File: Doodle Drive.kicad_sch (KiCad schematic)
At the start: 38 parts, among them J1 USB_B, J2 PINHD_1x4_Male, J3 Screw_Terminal_01x02, J6 PINHD_1x2_Male, J9 PINHD_1x3_Male, U1 STM32F411RETx, U6 AP7343-33W5-7, U7 CP2102-GMR, Y1 32.768KHz ±20ppm 12.5pF, Y2 25MHZ 12PF

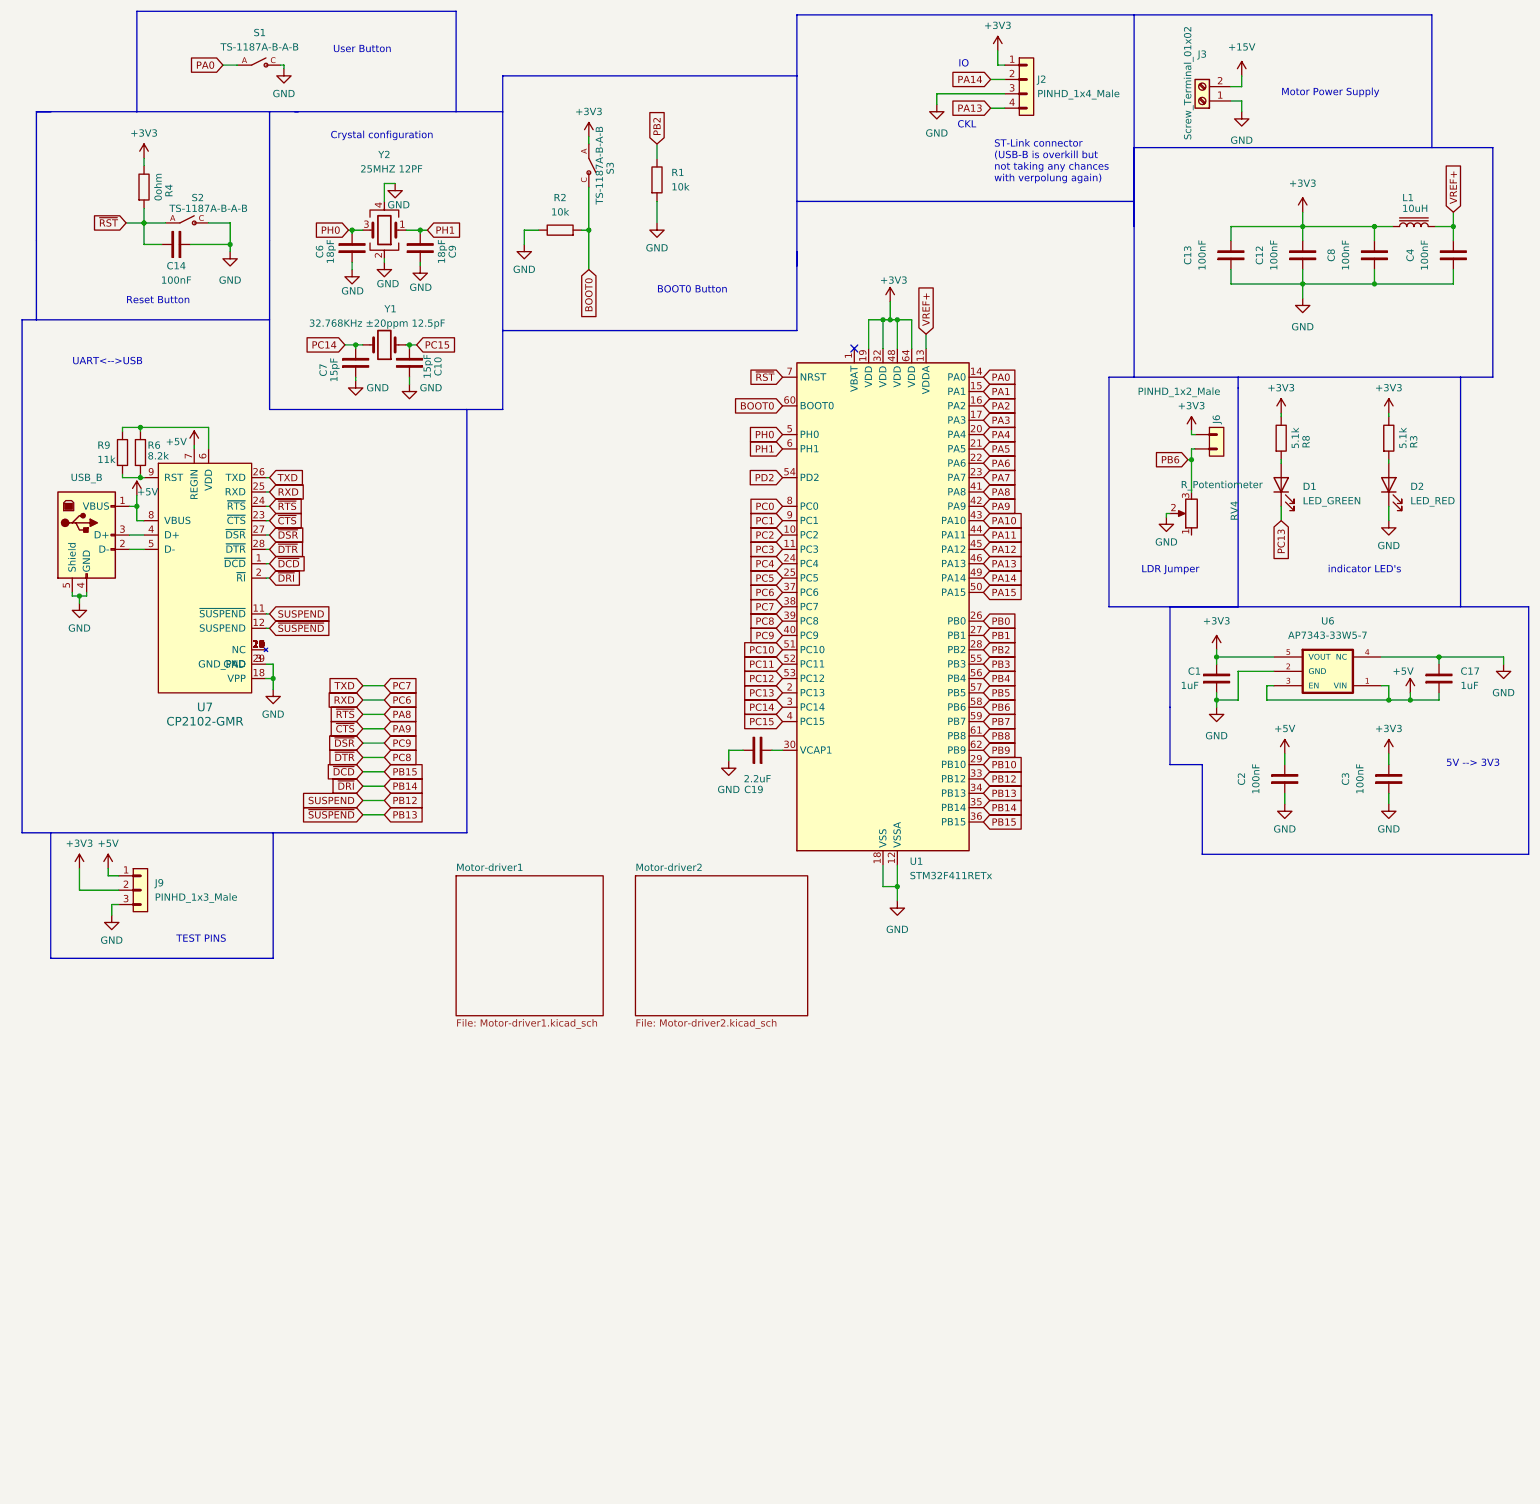
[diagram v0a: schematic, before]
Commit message: letzter code
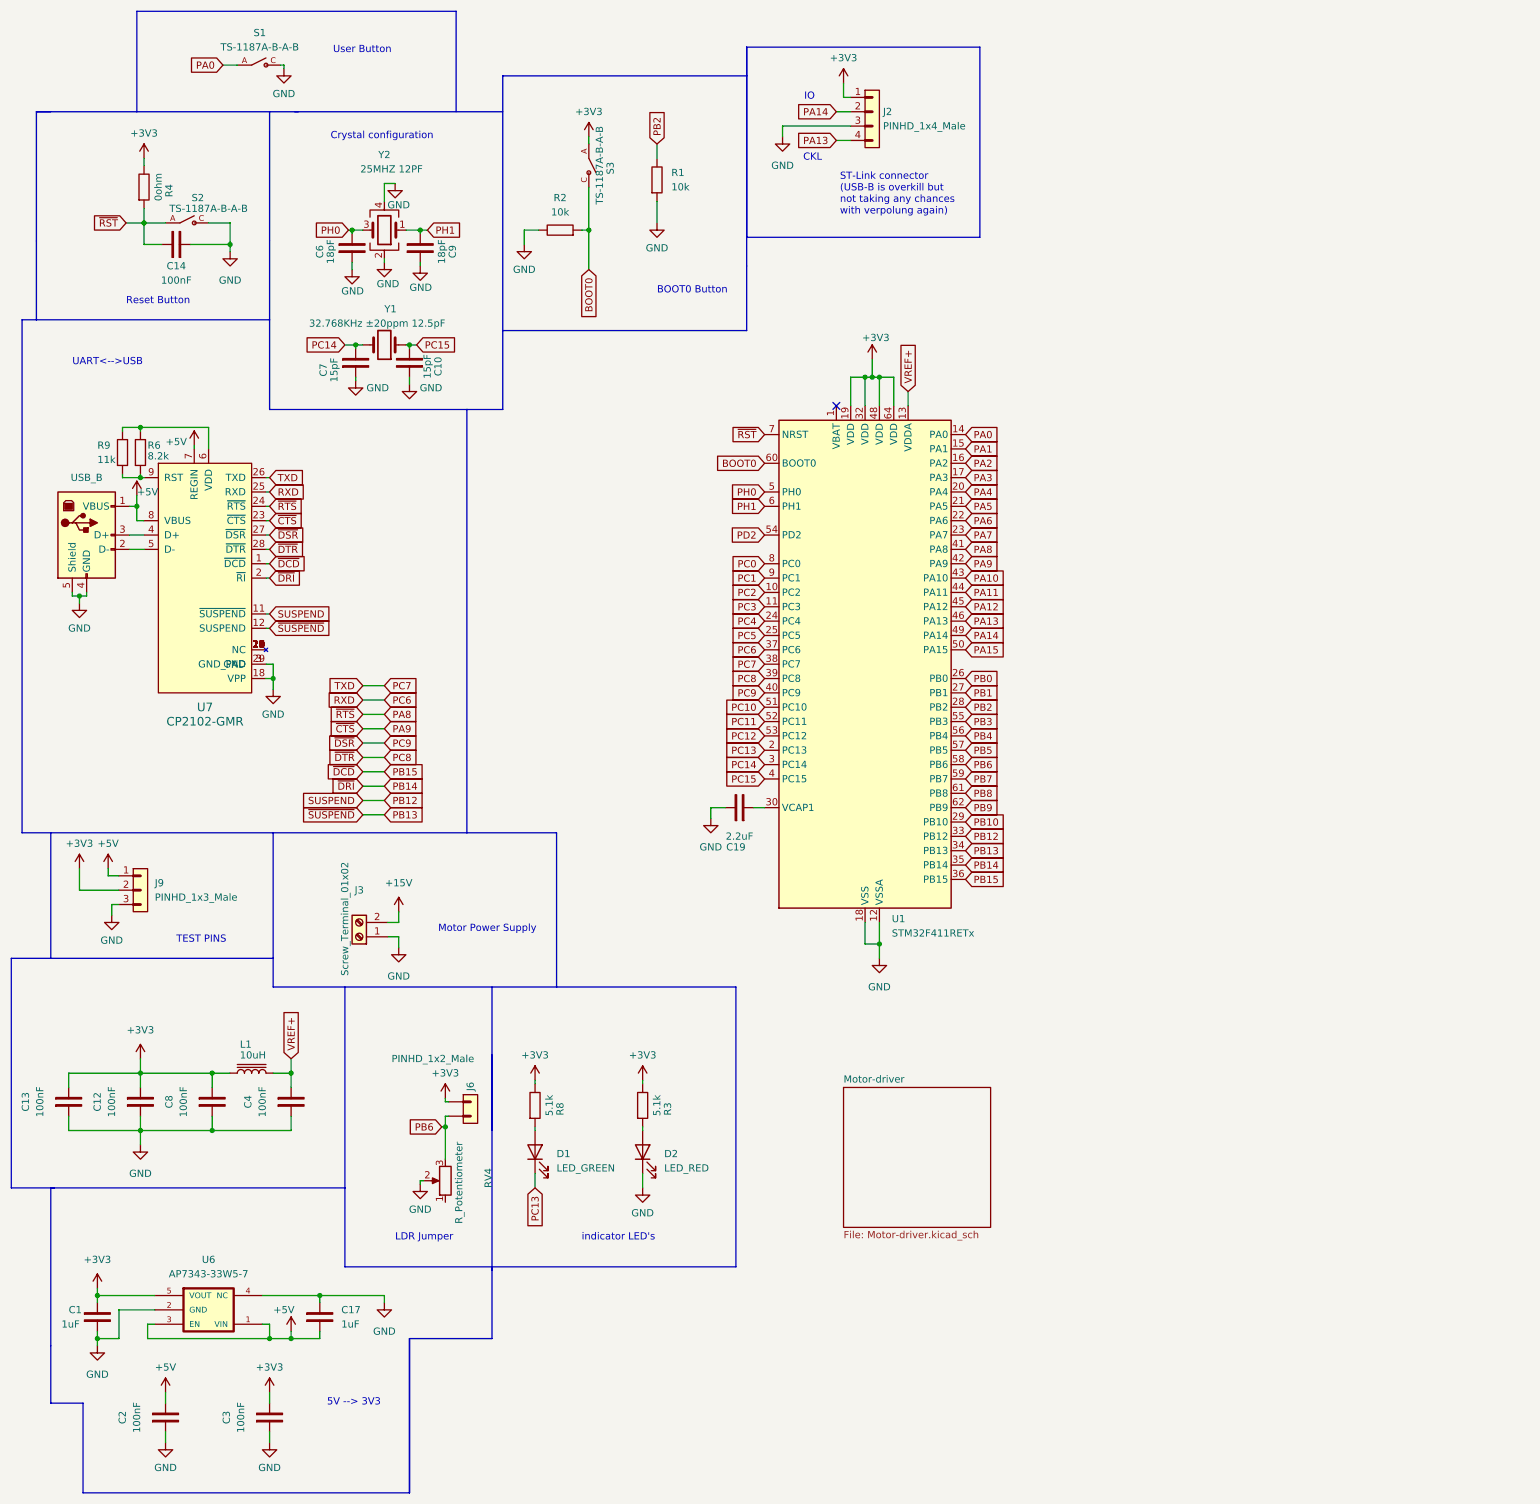
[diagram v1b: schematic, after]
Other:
- sheet Motor-driver1 renamed Motor-driver
- removed sheet Motor-driver2
- sheet Motor-driver: file Motor-driver1.kicad_sch -> Motor-driver.kicad_sch
- moved on the sheet: C1, C12, C13, C17, C19, C2, C3, C4, C8, D1, D2, J2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
